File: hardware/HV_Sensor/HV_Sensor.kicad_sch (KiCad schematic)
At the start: 28 parts, among them J1 Conn_01x09_Socket, J2 Conn_02x05_Odd_Even, J3 Conn_01x04_Pin, SW1 SW_Push, U2 MCU-MSM0G3507SPM, U4 AMC3330DWE

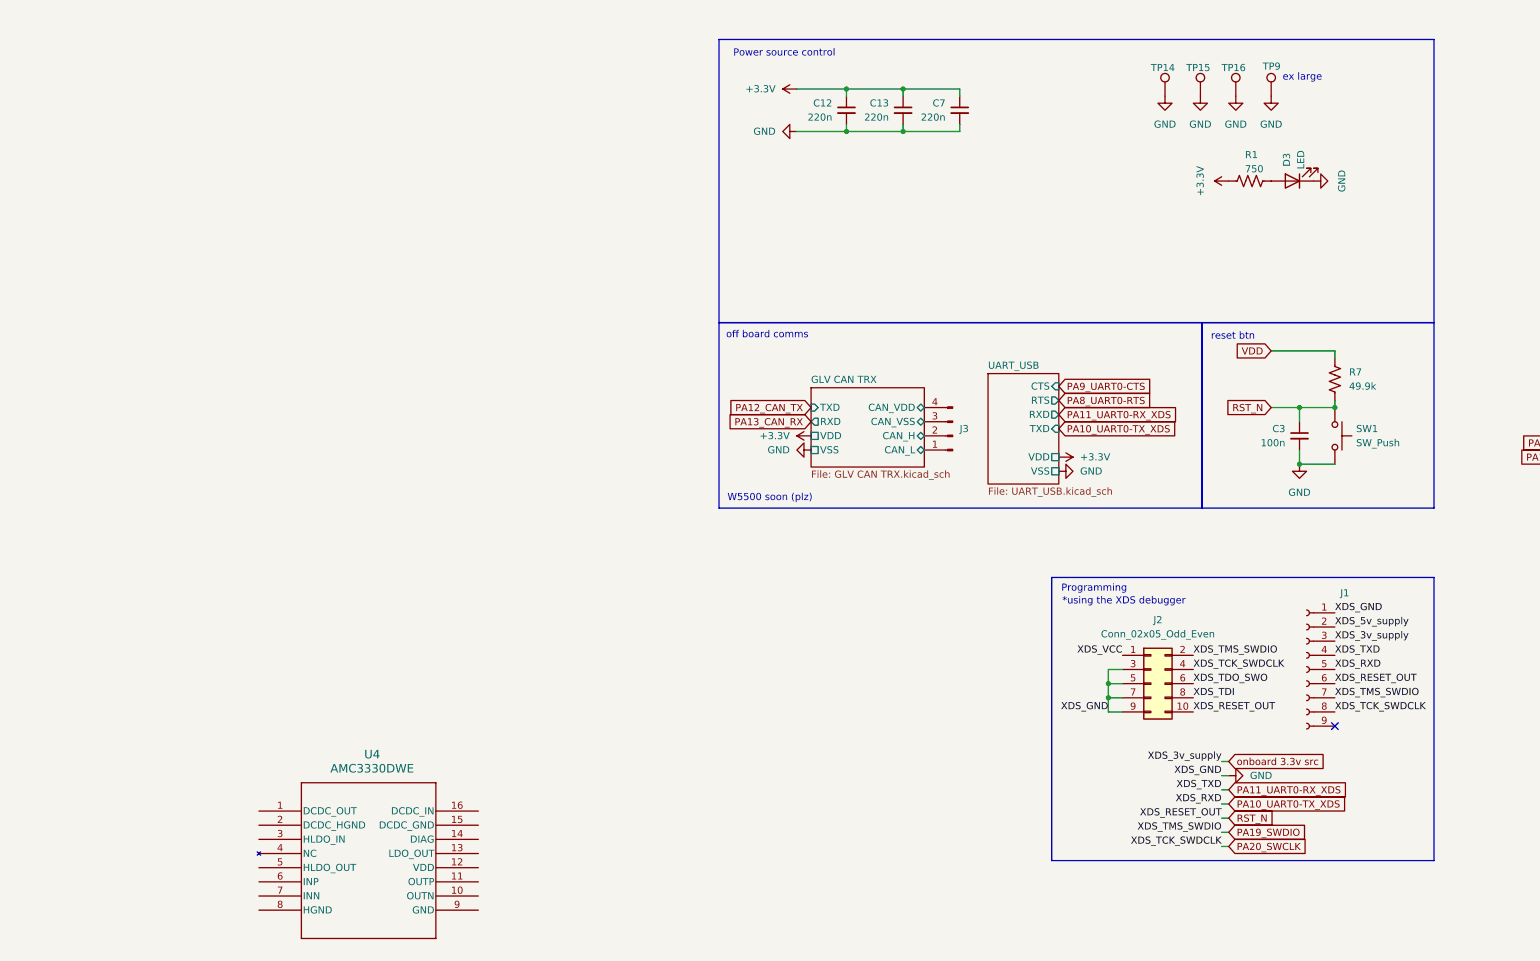
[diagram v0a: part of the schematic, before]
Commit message: lbjaeckbjaebjl
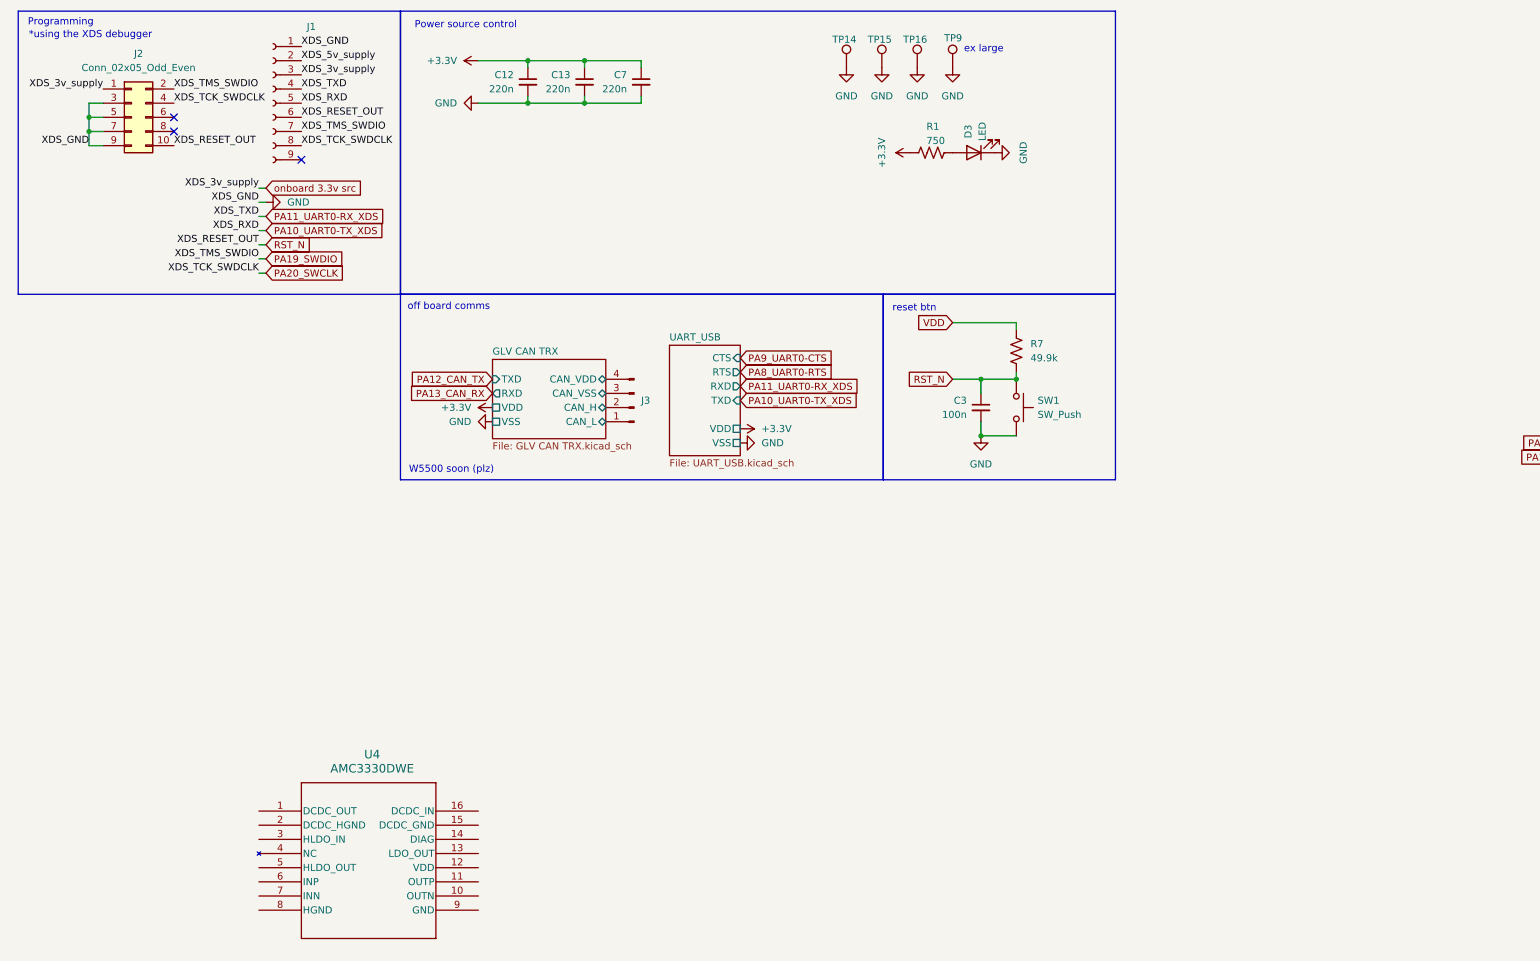
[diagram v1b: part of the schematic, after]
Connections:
- net XDS_VCC is gone; now on net onboard 3.3v src: J2.1 (Pin_1)
- net XDS_TDI: no longer names the net of J2.8 (Pin_8)
- net XDS_TDO_SWO: no longer names the net of J2.6 (Pin_6)
- no-connect marks 45 -> 47
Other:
- moved on the sheet: C12, C13, C3, C7, D3, J1, J2, J3, R1, R7, SW1, TP14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
